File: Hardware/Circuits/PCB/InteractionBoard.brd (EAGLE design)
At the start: 72 x 150.1 mm, 98 parts, among them J1 2X6 FEMALE, J2 2X6 FEMALE, SW1 219-10, U1 SX1509, U2 SX1509, U4 SX1509

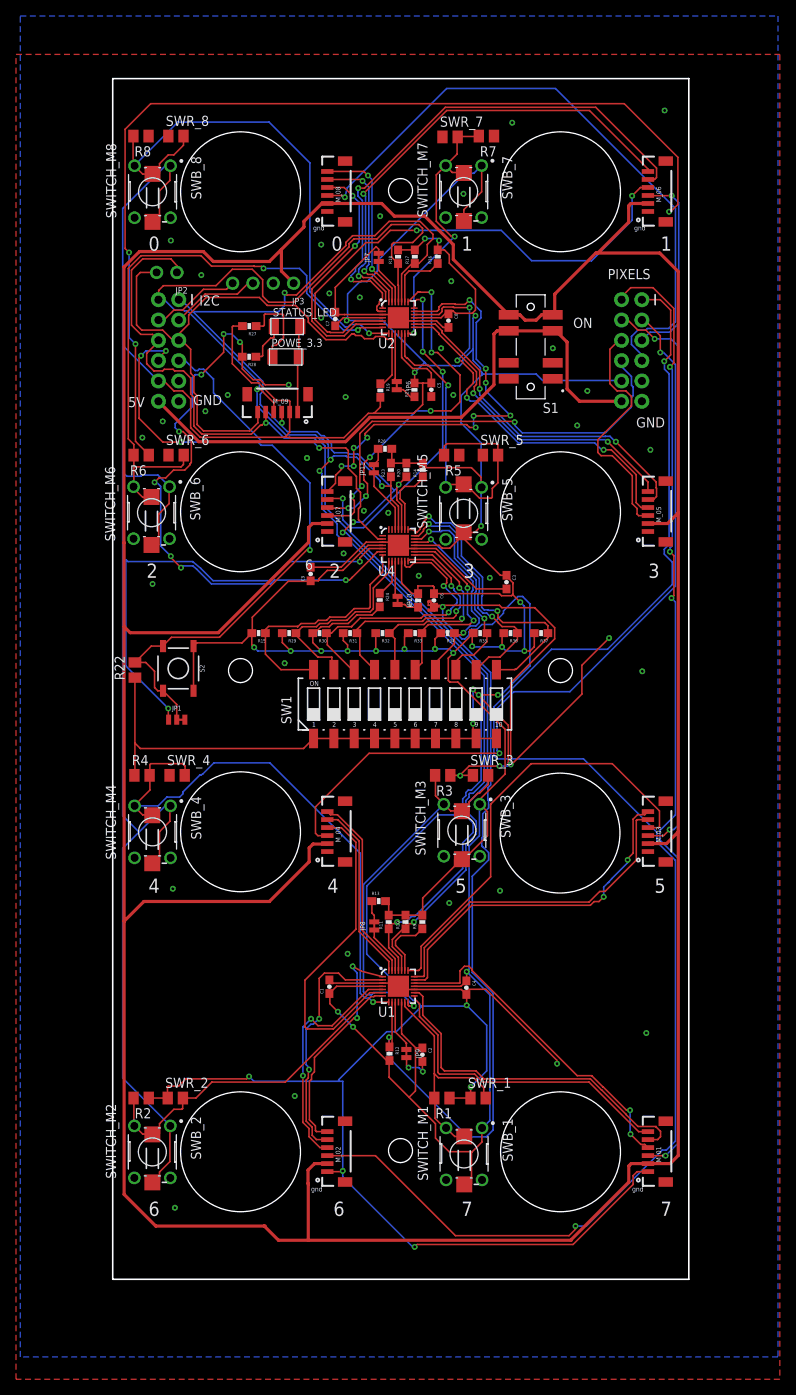
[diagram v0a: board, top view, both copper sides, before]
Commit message: update circuits
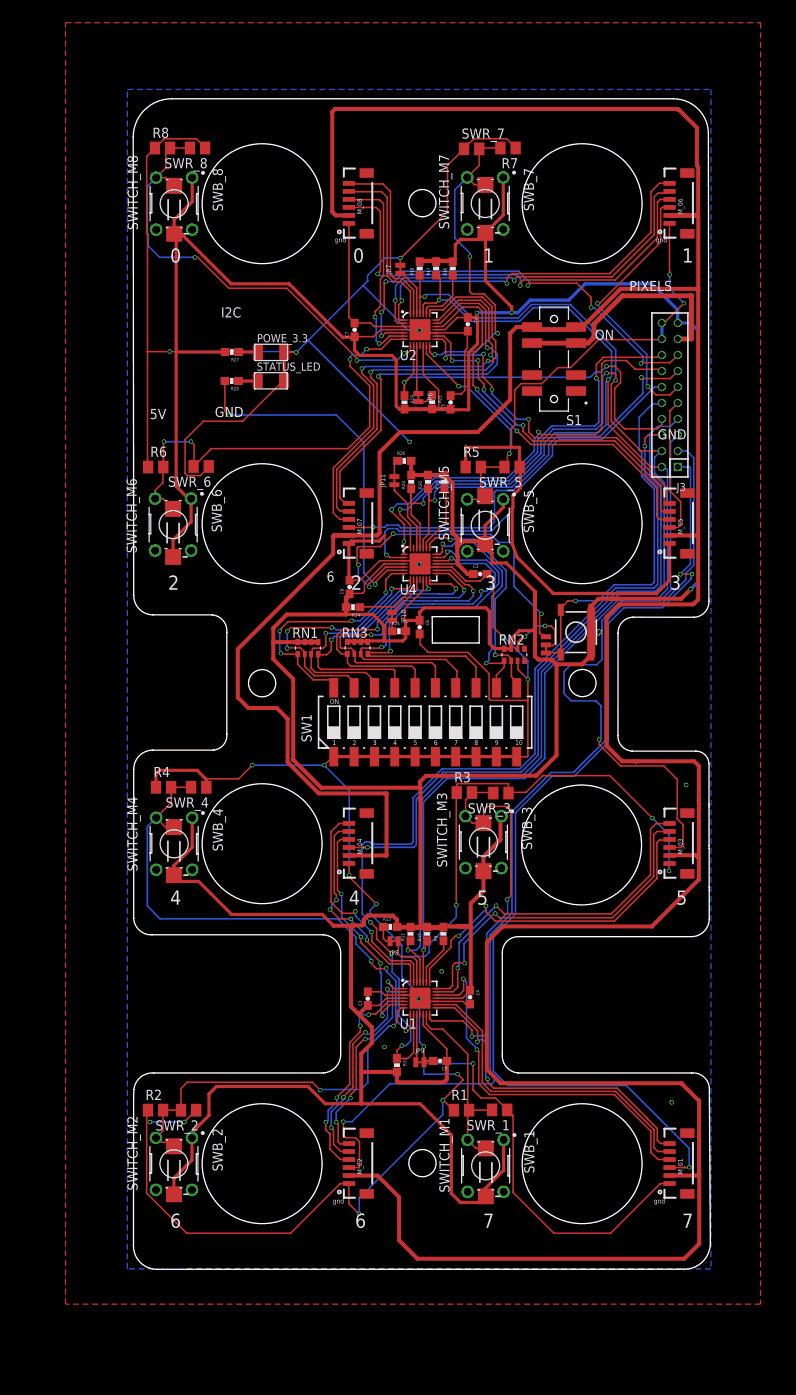
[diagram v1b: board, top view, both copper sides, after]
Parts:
- removed J1, J2: 2X6 FEMALE, SparkFun-Connectors:2X6
- removed JP2: (no value), microbuilder:1X02_ROUND
- removed JP3: (no value), microbuilder:1X04_ROUND
- removed M_09: (no value), SparkFun-Connectors:1X06-1MM
- removed R15, R29, R30, R31, R32, R33, R34, R35, R36, R37: 10K, SparkFun-Resistors:0603-RES
- removed R22: 10K, resistor:M0805
- added J3: F-2X10-DIL-2MM, con-headers-jp:DIL-2MM-2X10
- added RN1, RN2, RN3: (no value), resistor-dil:EXB38V
- moved S2 49.9 mm to (58.3, 80.8)
- moved JP1 47.1 mm to (54.5, 79.3), turned to 270 degrees
- moved STATUS_LED 7.08 mm to (20.1, 112.3)
- moved C9 5.14 mm to (30.0, 86.5)
- moved C1 5.03 mm to (32.2, 35.0)
- moved R25 4.54 mm to (36.1, 81.0), turned to 0 degrees
- moved R27 3.90 mm to (15.3, 115.9)
- moved C6 3.80 mm to (38.7, 81.5)
- moved R28 3.73 mm to (15.2, 112.2)
- moved U4 3.56 mm to (38.8, 89.4)
- moved R13 3.53 mm to (35.0, 44.0)
- moved R24 3.46 mm to (30.4, 84.0), turned to 180 degrees
- moved C3 3.45 mm to (46.3, 88.1), turned to 0 degrees
- moved R3 3.45 mm to (44.3, 60.8), turned to 0 degrees
- moved SWR_6 3.44 mm to (11.4, 101.6), turned to 180 degrees
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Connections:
- removed net CAN_RX2: J1.4, JP3.4
- removed net CAN_TX2: J1.3, JP3.3
- net 10_SX3: now also RN3.1; no longer R32.1
- net 11_SX3: now also RN3.2; no longer R33.1
- net 12_SX3: now also RN3.3; no longer R34.1
- net 13_SX3: now also RN3.4; no longer R35.1
- net 14_SX3: now also RN2.1; no longer R36.1
- net 15_SX3: now also RN2.2; no longer R37.1
- net 1_SX3: now also J3.16
- net 2_SX3: now also J3.14
- net 3.3V: now also J3.19, RN1.5, RN1.6, RN1.7, RN1.8, RN2.7, RN2.8, RN3.5, RN3.6, RN3.7, RN3.8; no longer J1.10, J2.10, M_09.2, R15.2, R29.2, R30.2, R31.2, R32.2, R33.2, R34.2, R35.2, R36.2, R37.2
- net 3_SX3: now also J3.12; no longer J1.7
- net 6_SX3: now also RN1.1; no longer R15.1
- net 7_SX3: now also RN1.2; no longer R29.1
- net 8_SX3: now also RN1.3; no longer R30.1
- net 9_SX3: now also RN1.4; no longer R31.1
- net GND_MCU: now also J3.18, J3.20, RN2.3; no longer J1.11, J1.9, J2.11, J2.9, JP3.2, M_09.1, R22.1
- net INT_01: now also J3.6; no longer J1.6, JP2.1, M_09.5
- net INT_02: now also J3.8; no longer J1.5, JP2.2, M_09.6
- net NEOPIXEL_01: now also J3.1; no longer J2.2
- net NEOPIXEL_02: now also J3.3; no longer J2.1
- net NEOPIXEL_03: now also J3.5; no longer J2.4
- net NEOPIXEL_04: now also J3.7; no longer J2.3
- net NEOPIXEL_05: now also J3.9; no longer J2.6
- net NEOPIXEL_06: now also J3.11; no longer J2.5
- net NEOPIXEL_07: now also J3.13; no longer J2.8
- net NEOPIXEL_08: now also J3.15; no longer J2.7
- net RESET: now also J3.10, RN2.6; no longer J1.8, R22.2
- net SCL_00: now also J3.4; no longer J1.2, M_09.4
- net SDA_00: now also J3.2; no longer J1.1, M_09.3
- net VCC_5V: no longer JP3.1
- net VCC_5V_IN: now also J3.17; no longer J1.12, J2.12
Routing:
- net GND_MCU: track 581.9 -> 682.2 mm, vias 58 -> 29
- net NEOPIXEL_02: track 191.1 -> 125.1 mm, vias 2 -> 1
- net INT_01: track 178.6 -> 118.8 mm, vias 2 -> 4
- net 2_SX3: track 0.00 -> 54.4 mm, vias 0 -> 3
- net 1_SX3: track 0.00 -> 51.7 mm, vias 0 -> 2
- net VCC_5V_IN: track 77.4 -> 30.4 mm
- net 5_SX3: track 78.5 -> 45.6 mm, vias 9 -> 2
- net 3.3V: track 718.7 -> 747.8 mm, vias 21 -> 3
- net RESET: track 85.3 -> 56.5 mm, vias 4 -> 3
- net INT_02: track 77.3 -> 50.0 mm, vias 0 -> 2
- net 12_SX3: track 24.6 -> 47.8 mm, vias 2 -> 3
- net 13_SX3: track 26.8 -> 50.0 mm
- net NEOPIXEL_08: track 80.0 -> 57.9 mm, vias 1 -> 4
- net 3_SX2: track 67.1 -> 47.9 mm
- net 11_SX3: track 25.4 -> 43.7 mm
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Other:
- board size 72 x 150.1 mm -> 72.1 x 146.3 mm
